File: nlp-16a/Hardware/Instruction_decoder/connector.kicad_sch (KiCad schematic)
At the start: 0 parts

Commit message: 命令デコーダ ロジック部の設計だいたい完了git statusgit statusやったぜ
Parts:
- added J? (x2): Conn_02x10_Odd_Even, Connector_PinHeader_2.54mm:PinHeader_2x10_P2.54mm_Horizontal, symbol Connector_Generic:Conn_02x10_Odd_Even
- added J? (x2): Conn_02x10_Counter_Clockwise, Connector_PinHeader_2.54mm:PinHeader_2x10_P2.54mm_Horizontal, symbol Connector_Generic:Conn_02x10_Odd_Even
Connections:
- new net 3word: J?.20 (Pin_20)
- new net ALL_CLK: J?.14 (Pin_14)
- new net A_BUS_Addr0: J?.2 (Pin_2), J?.20 (Pin_20)
- new net A_BUS_Addr1: J?.18 (Pin_18), J?.4 (Pin_4)
- new net A_BUS_Addr2: J?.16 (Pin_16), J?.6 (Pin_6)
- new net A_BUS_Addr3: J?.14 (Pin_14), J?.8 (Pin_8)
- new net BUS_A/~{B}: J?.9 (Pin_9)
- new net BUS_A/~{Y}: J?.7 (Pin_7)
- new net Fetch: J?.11 (Pin_11)
- new net GND: J?.16 (Pin_16), J?.16 (Pin_16), J?.18 (Pin_18), J?.18 (Pin_18), J?.20 (Pin_20), J?.20 (Pin_20)
- new net INT: J?.16 (Pin_16)
- new net OP0: J?.19 (Pin_19)
- new net OP1: J?.17 (Pin_17)
- new net OP2: J?.15 (Pin_15)
- new net OP3: J?.13 (Pin_13)
- new net OP4: J?.11 (Pin_11)
- new net OP5: J?.9 (Pin_9)
- new net OP6: J?.7 (Pin_7)
- new net OP7: J?.5 (Pin_5)
- new net RS: J?.14 (Pin_14)
- new net Seed_pluse: J?.12 (Pin_12)
- new net Y_BUS_Addr0: J?.12 (Pin_12), J?.2 (Pin_2)
- new net Y_BUS_Addr1: J?.10 (Pin_10), J?.4 (Pin_4)
- new net Y_BUS_Addr2: J?.6 (Pin_6), J?.8 (Pin_8)
- new net Y_BUS_Addr3: J?.6 (Pin_6), J?.8 (Pin_8)
- new net Y_Flag_sel: J?.13 (Pin_13)
- new net phi1: J?.12 (Pin_12)
- new net phi2: J?.10 (Pin_10)
- new net ~{Acc_Y}: J?.13 (Pin_13)
- new net ~{Address_Y}: J?.5 (Pin_5)
- new net ~{DEC_ALU}: J?.15 (Pin_15)
- new net ~{Flag_A}: J?.9 (Pin_9)
- new net ~{Flag_Y}: J?.9 (Pin_9)
- new net ~{INC_ALU}: J?.17 (Pin_17)
- new net ~{INTERNAL_ALU}: J?.19 (Pin_19)
- new net ~{INTERNAL_A}: J?.19 (Pin_19)
- new net ~{INTERNAL_Y}: J?.19 (Pin_19)
- new net ~{IP_A}: J?.3 (Pin_3)
- new net ~{IP_Y}: J?.3 (Pin_3)
- new net ~{IR1_Y}: J?.17 (Pin_17)
- new net ~{IR2_Y}: J?.15 (Pin_15)
- new net ~{IR3_Y}: J?.11 (Pin_11)
- new net ~{IV_A}: J?.13 (Pin_13)
- new net ~{MEM_A}: J?.7 (Pin_7)
- new net ~{MEM_Y}: J?.7 (Pin_7)
- new net ~{NOP}: J?.18 (Pin_18)
- new net ~{SP_A}: J?.1 (Pin_1)
- new net ~{SP_Y}: J?.1 (Pin_1)
- no-connect marks 0 -> 7
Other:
- note added: "YバスではΦ1，Φ2で使用する"
- note added: "Yバスでは全レジスタ指定で使用する"

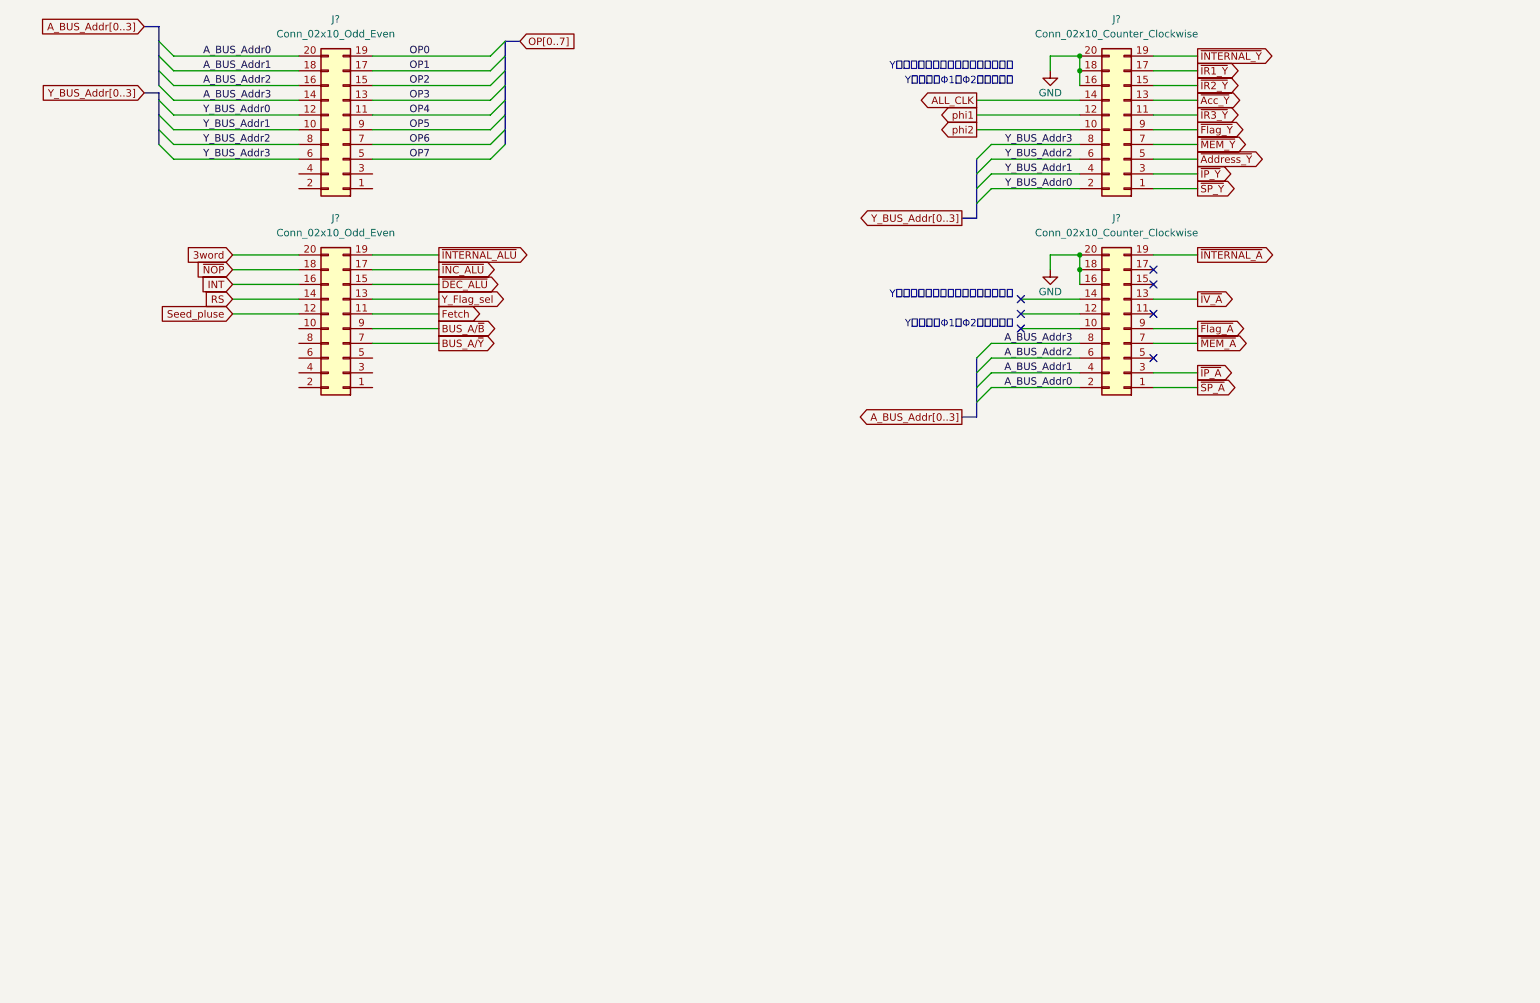
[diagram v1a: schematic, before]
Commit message: アノテーションまで完了．基板設計に入る
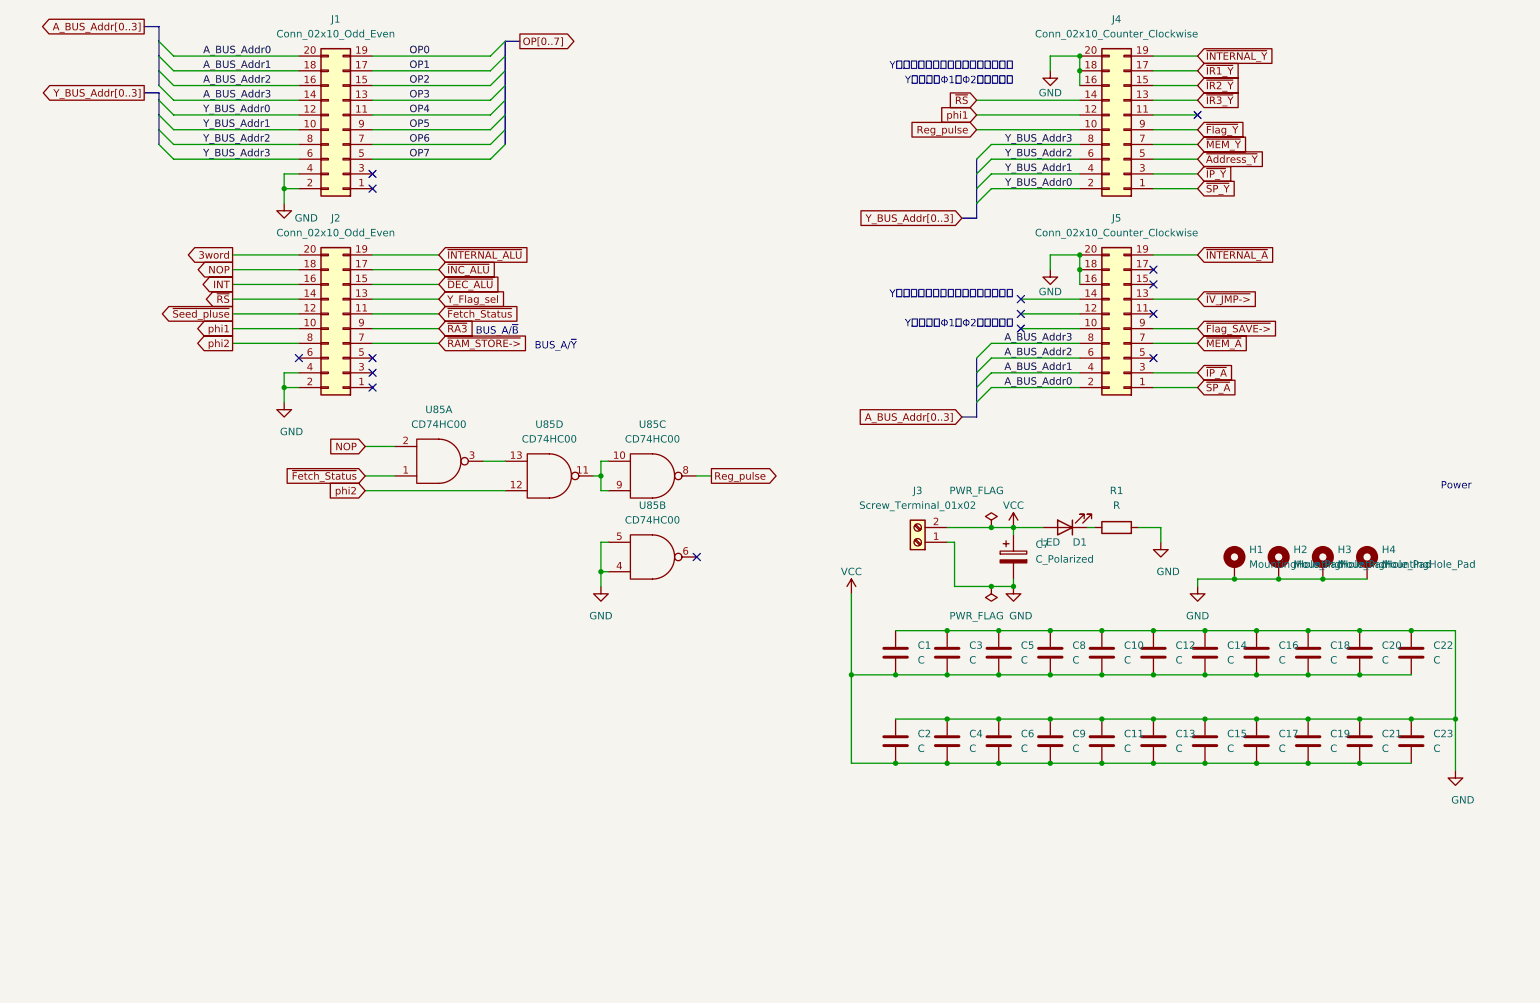
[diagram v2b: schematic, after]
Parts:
- added C1, C10, C11, C12, C13, C14, C15, C16, C17, C18, C19, C2, C20, C21, C22, C23, C3, C4, C5, C6, C8, C9: C, Capacitor_THT:C_Disc_D7.5mm_W2.5mm_P5.00mm, symbol Device:C
- added C7: C_Polarized, Capacitor_THT:CP_Radial_D5.0mm_P2.50mm, symbol Device:C_Polarized
- added D1: LED, LED_THT:LED_D3.0mm, symbol Device:LED
- added H1, H2, H3, H4: MountingHole_Pad, MountingHole:MountingHole_3mm_Pad, symbol Mechanical:MountingHole_Pad
- added J3: Screw_Terminal_01x02, TerminalBlock:TerminalBlock_bornier-2_P5.08mm, symbol Connector:Screw_Terminal_01x02
- added R1: R, Resistor_SMD:R_0603_1608Metric_Pad0.98x0.95mm_HandSolder, symbol Device:R
- added U85: CD74HC00, Package_DIP:DIP-14_W7.62mm, symbol CD74HCXX:CD74HC00
- gave numbers to parts that had none: 4
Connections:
- net RS is gone; now on net ~{RS}: J2.14 (Pin_14)
- net ~{Acc_Y} is gone; now on net ~{IR3_Y}: J4.13 (Pin_13)
- net GND: now also J1.2 (Pin_2), J1.4 (Pin_4), J2.2 (Pin_2), J2.4 (Pin_4), C1.1, C10.1, C11.1, C12.1, C13.1, C14.1, C15.1, C16.1, C17.1, C18.1, C19.1, C2.1, C20.1, C21.1, C22.1, C23.1, C3.1, C4.1, C5.1, C6.1, C7.2, C8.1, C9.1, H1.1, H2.1, H3.1, H4.1, J3.1 (Pin_1), R1.2, U85.4, U85.5, U85.7 (GND), U85.7 (GND), U85.7 (GND), U85.7 (GND)
- net phi1: now also J2.10 (Pin_10)
- net phi2: now also J2.8 (Pin_8), U85.12; no longer J4.10 (Pin_10)
- net ~{IR3_Y}: no longer J4.11 (Pin_11)
- net ALL_CLK renamed ~{RS}
- net BUS_A/~{B} renamed ~{RA3}
- net BUS_A/~{Y} renamed ~{RAM_STORE->}
- net Fetch renamed ~{Fetch_Status}
- net ~{Fetch_Status}: now also U85.1
- net Seed_pluse renamed ~{Seed_pluse}
- net ~{Flag_A} renamed ~{Flag_SAVE->}
- net ~{IV_A} renamed ~{IV_JMP->}
- net ~{NOP} renamed NOP
- net NOP: now also U85.2
- new net: D1.1 (K), R1.1
- new net: U85.13, U85.3
- new net: U85.10, U85.11, U85.9
- new net Reg_pulse: J4.10 (Pin_10), U85.8
- new net VCC: C1.2, C10.2, C11.2, C12.2, C13.2, C14.2, C15.2, C16.2, C17.2, C18.2, C19.2, C2.2, C20.2, C21.2, C22.2, C23.2, C3.2, C4.2, C5.2, C6.2, C7.1, C8.2, C9.2, D1.2 (A), J3.2 (Pin_2), U85.14 (VCC), U85.14 (VCC), U85.14 (VCC), U85.14 (VCC)
- no-connect marks 7 -> 15
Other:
- note added: "BUS_A/~{B}"
- note added: "BUS_A/~{Y}"
- note added: "Power"

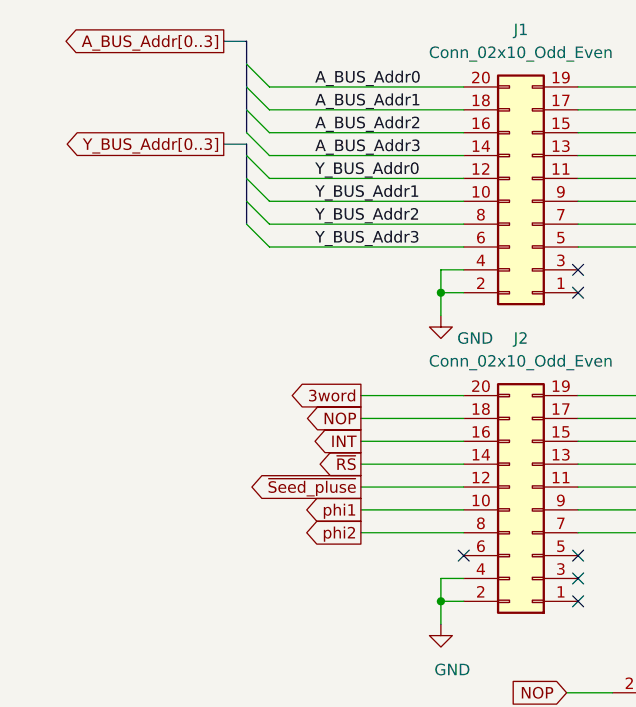
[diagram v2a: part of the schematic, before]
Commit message: 基板設計 今日はとりあえずここまで
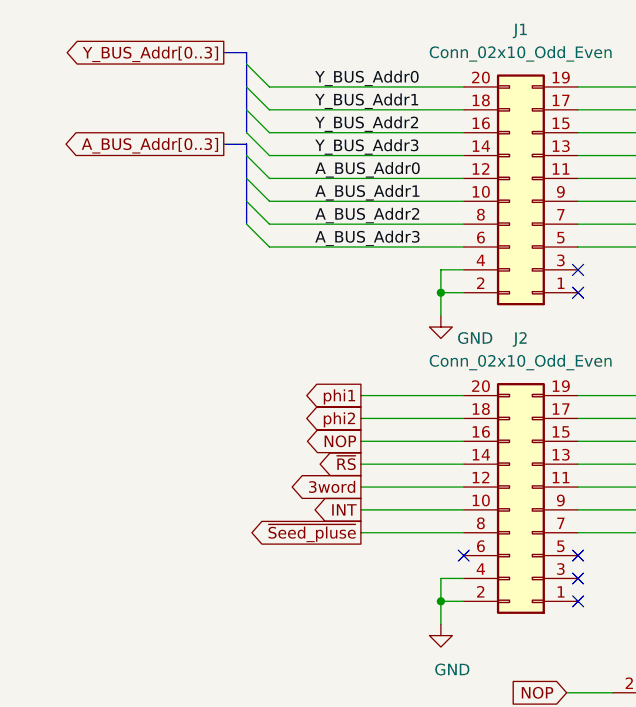
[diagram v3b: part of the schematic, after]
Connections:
- net 3word: now also J2.12 (Pin_12); no longer J2.20 (Pin_20)
- net A_BUS_Addr0: now also J1.12 (Pin_12); no longer J1.20 (Pin_20)
- net A_BUS_Addr1: now also J1.10 (Pin_10); no longer J1.18 (Pin_18)
- net A_BUS_Addr2: now also J1.8 (Pin_8); no longer J1.16 (Pin_16)
- net A_BUS_Addr3: now also J1.6 (Pin_6); no longer J1.14 (Pin_14)
- net INT: now also J2.10 (Pin_10); no longer J2.16 (Pin_16)
- net NOP: now also J2.16 (Pin_16); no longer J2.18 (Pin_18)
- net Y_BUS_Addr0: now also J1.20 (Pin_20); no longer J1.12 (Pin_12)
- net Y_BUS_Addr1: now also J1.18 (Pin_18); no longer J1.10 (Pin_10)
- net Y_BUS_Addr2: now also J1.16 (Pin_16); no longer J1.8 (Pin_8)
- net Y_BUS_Addr3: now also J1.14 (Pin_14); no longer J1.6 (Pin_6)
- net phi1: now also J2.20 (Pin_20); no longer J2.10 (Pin_10)
- net phi2: now also J2.18 (Pin_18); no longer J2.8 (Pin_8)
- net ~{Seed_pluse}: now also J2.8 (Pin_8); no longer J2.12 (Pin_12)

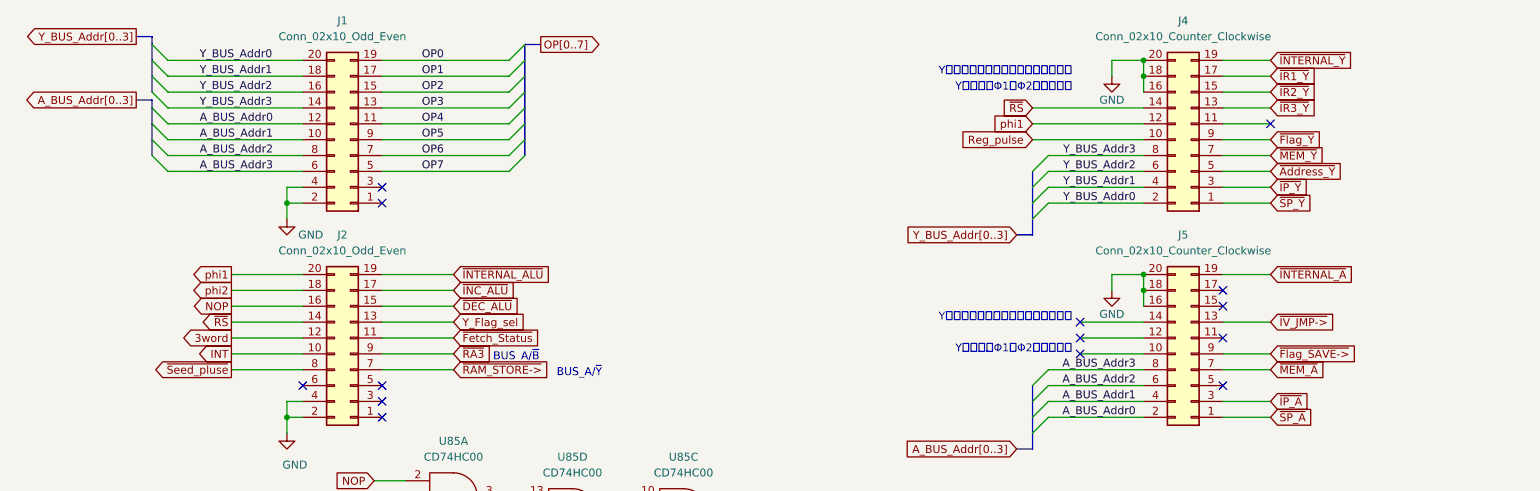
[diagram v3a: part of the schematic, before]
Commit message: 基板設計 進捗
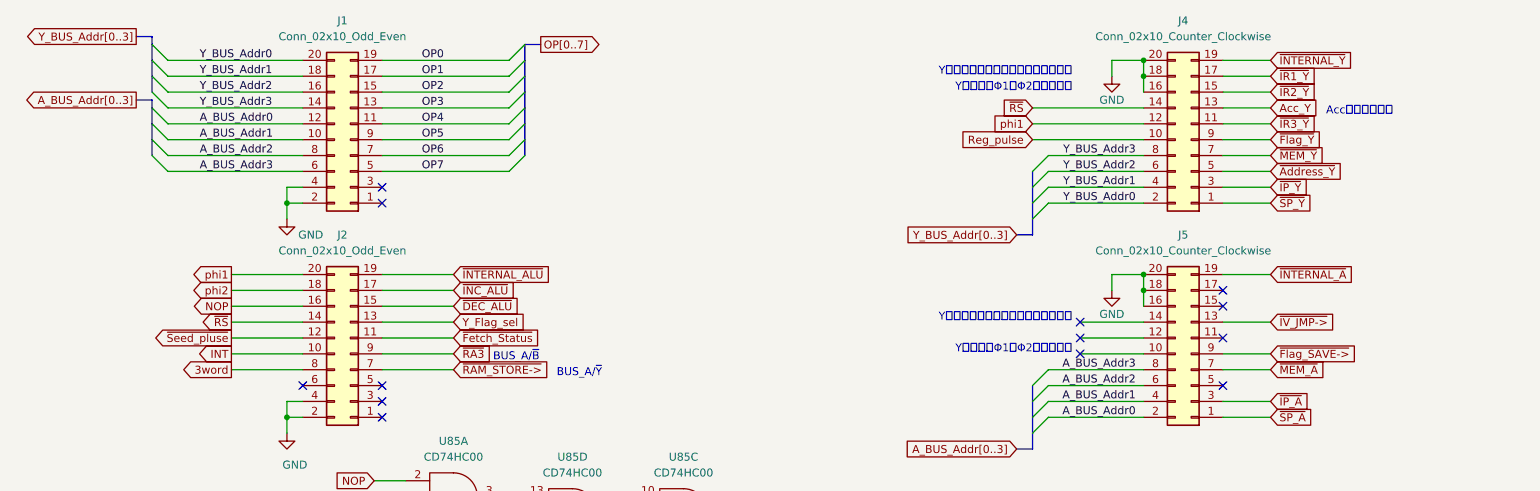
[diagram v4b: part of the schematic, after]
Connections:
- net 3word: now also J2.8 (Pin_8); no longer J2.12 (Pin_12)
- net ~{IR3_Y}: now also J4.11 (Pin_11); no longer J4.13 (Pin_13)
- net ~{Seed_pluse}: now also J2.12 (Pin_12); no longer J2.8 (Pin_8)
- new net Acc_Y: J4.13 (Pin_13)
- no-connect marks 15 -> 14
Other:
- note added: "Accだけは正論理"
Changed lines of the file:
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@@
   (junction (at 168.91 142.24) (diameter 0) (color 0 0 0 0)
   )
-  (no_connect (at 228.6 45.72))
   (no_connect (at 142.24 121.92))
   (no_connect (at 73.66 87.63))
@@
     (effects (font (size 1.27 1.27)) (justify left bottom))
   )
+  (text "Accだけは正論理" (at 237.49 44.45 0)
+    (effects (font (size 1.27 1.27)) (justify left bottom))
+  )
   (text "BUS_A/~{B}" (at 104.14 83.82 0)
     (effects (font (size 1.27 1.27)) (justify left bottom))
@@
     )
   )
-  (global_label "~{Seed_pluse}" (shape output) (at 62.23 85.09 180) (fields_autoplaced)
-    (effects (font (size 1.27 1.27)) (justify right))
-    (property "Intersheet References" "${INTERSHEET_REFS}" (id 0) (at 49.2336 85.0106 0)
+  (global_label "~{Seed_pluse}" (shape output) (at 62.23 80.01 180) (fields_autoplaced)
+    (effects (font (size 1.27 1.27)) (justify right))
+    (property "Intersheet References" "${INTERSHEET_REFS}" (id 0) (at 49.2336 79.9306 0)
       (effects (font (size 1.27 1.27)) (justify right) hide)
     )
@@
     )
   )
-  (global_label "~{IR3_Y}" (shape input) (at 228.6 43.18 0) (fields_autoplaced)
-    (effects (font (size 1.27 1.27)) (justify left))
-    (property "Intersheet References" "${INTERSHEET_REFS}" (id 0) (at 236.1536 43.1006 0)
+  (global_label "~{IR3_Y}" (shape input) (at 228.6 45.72 0) (fields_autoplaced)
+    (effects (font (size 1.27 1.27)) (justify left))
+    (property "Intersheet References" "${INTERSHEET_REFS}" (id 0) (at 236.1536 45.6406 0)
       (effects (font (size 1.27 1.27)) (justify left) hide)
     )
@@
     )
   )
+  (global_label "Acc_Y" (shape input) (at 228.6 43.18 0) (fields_autoplaced)
+    (effects (font (size 1.27 1.27)) (justify left))
+    (property "Intersheet References" "${INTERSHEET_REFS}" (id 0) (at 236.335 43.1006 0)
+      (effects (font (size 1.27 1.27)) (justify left) hide)
+    )
+  )
   (global_label "~{SP_Y}" (shape input) (at 228.6 58.42 0) (fields_autoplaced)
     (effects (font (size 1.27 1.27)) (justify left))
@@
     )
   )
-  (global_label "3word" (shape output) (at 62.23 80.01 180) (fields_autoplaced)
-    (effects (font (size 1.27 1.27)) (justify right))
-    (property "Intersheet References" "${INTERSHEET_REFS}" (id 0) (at 54.1926 79.9306 0)
-      (effects (font (size 1.27 1.27)) (justify right) hide)
-    )
+  (global_label "3word" (shape output) (at 62.23 85.09 180) (fields_autoplaced)
+    (effects (font (size 1.27 1.27)) (justify right))
+    (property "Intersheet References" "${INTERSHEET_REFS}" (id 0) (at 54.1926 85.0106 0)
+      (effects (font (size 1.27 1.27)) (justify right) hide)
+    )
